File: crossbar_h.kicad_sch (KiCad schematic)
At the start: 64 parts, among them U100 AD5160, U101 AD5160, U102 AD5160, U103 AD5160, U104 AD5160, U105 AD5160, U106 AD5160, U107 AD5160, U108 AD5160, U109 AD5160, U110 AD5160, U111 AD5160, U112 AD5160, U113 AD5160, U114 AD5160, U115 AD5160, U116 AD5160, U117 AD5160, U118 AD5160, U119 AD5160, U120 AD5160, U121 AD5160, U122 AD5160, U123 AD5160, U124 AD5160, U125 AD5160, U126 AD5160, U127 AD5160, U128 AD5160, U129 AD5160, U130 AD5160, U131 AD5160

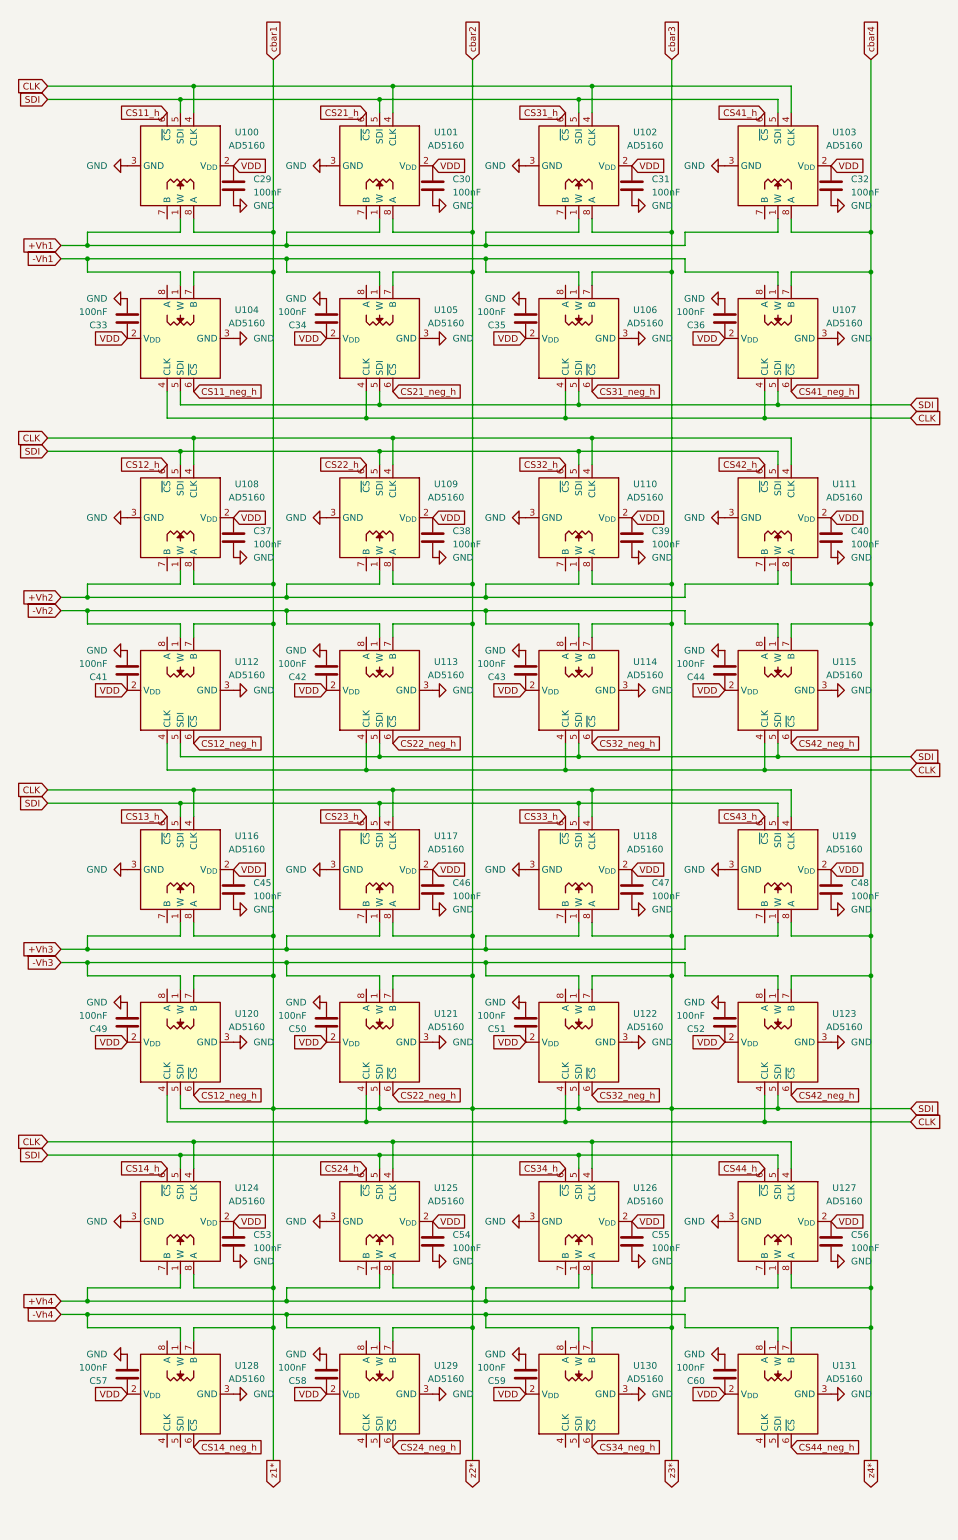
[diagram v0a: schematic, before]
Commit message: Updated: power
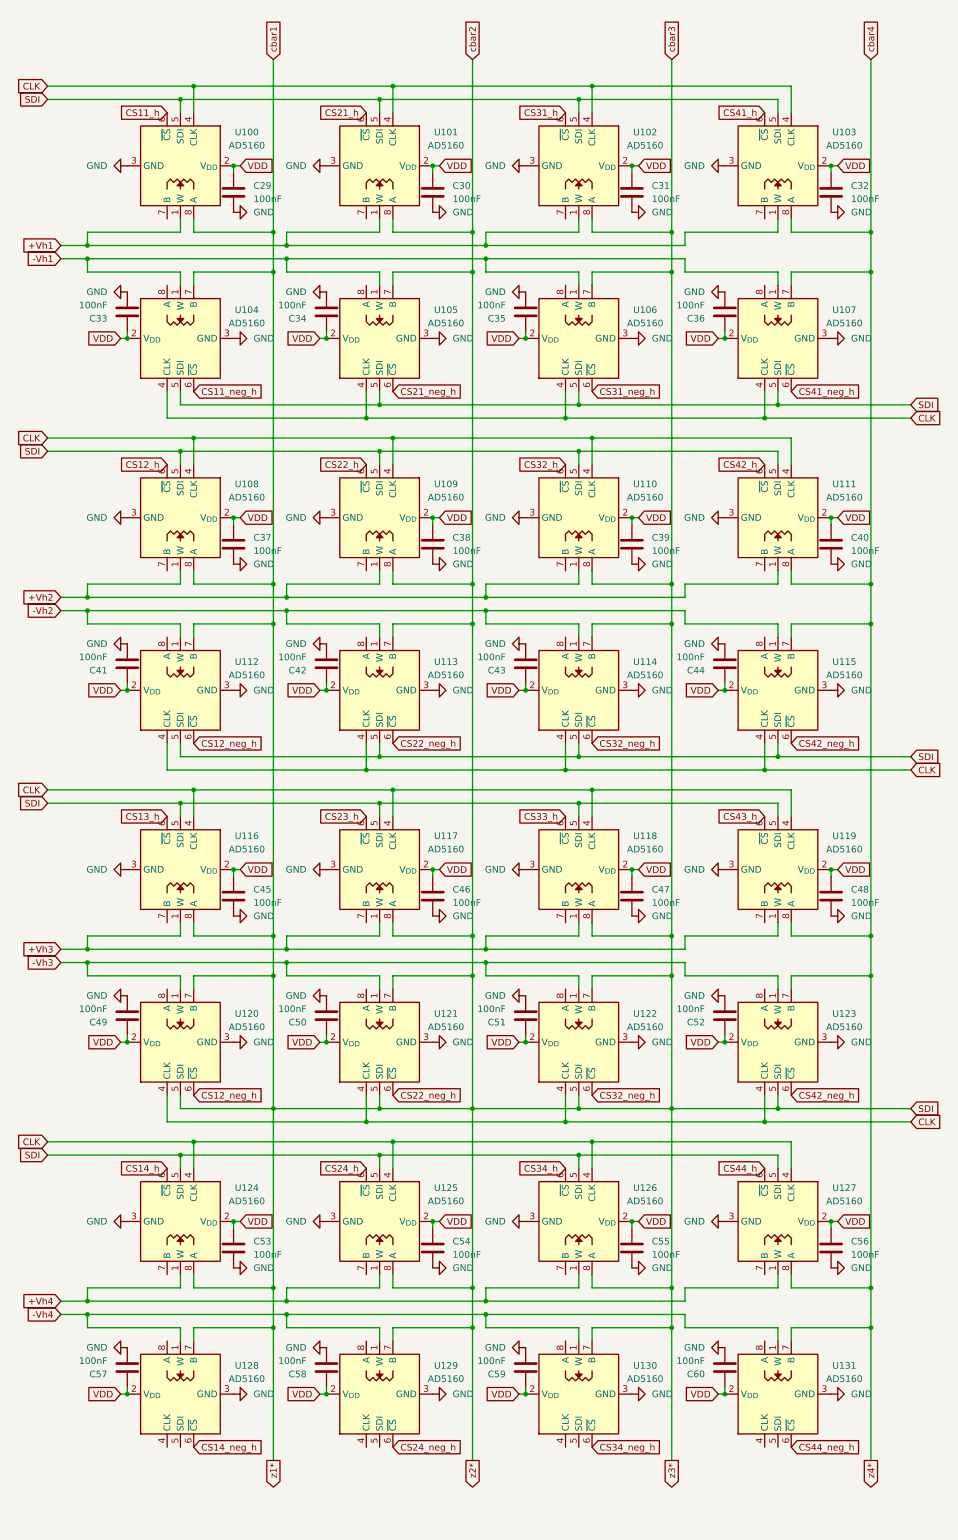
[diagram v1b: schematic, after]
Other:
- moved on the sheet: C29

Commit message: Updated: op amps
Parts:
- C29, C30, C31, C32, C33, C34, C35, C36, C37, C38, C39, C40, C41, C42, C43, C44, C45, C46, C47, C48, C49, C50, C51, C52, C53, C54, C55, C56, C57, C58, C59, C60: footprint (none) -> Capacitor_SMD:C_1206_3216Metric_Pad1.33x1.80mm_HandSolder
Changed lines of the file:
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@@
 			)
 		)
-		(property "Footprint" ""
+		(property "Footprint" "Capacitor_SMD:C_1206_3216Metric_Pad1.33x1.80mm_HandSolder"
 			(at 199.6948 240.03 0)
 			(effects
@@
 			)
 		)
-		(property "Footprint" ""
+		(property "Footprint" "Capacitor_SMD:C_1206_3216Metric_Pad1.33x1.80mm_HandSolder"
 			(at 221.9452 224.79 0)
 			(effects
@@
 			)
 		)
-		(property "Footprint" ""
+		(property "Footprint" "Capacitor_SMD:C_1206_3216Metric_Pad1.33x1.80mm_HandSolder"
 			(at 107.6452 90.17 0)
 			(effects
@@
 			)
 		)
-		(property "Footprint" ""
+		(property "Footprint" "Capacitor_SMD:C_1206_3216Metric_Pad1.33x1.80mm_HandSolder"
 			(at 199.6948 307.34 0)
 			(effects
@@
 			)
 		)
-		(property "Footprint" ""
+		(property "Footprint" "Capacitor_SMD:C_1206_3216Metric_Pad1.33x1.80mm_HandSolder"
 			(at 123.4948 240.03 0)
 			(effects
@@
 			)
 		)
-		(property "Footprint" ""
+		(property "Footprint" "Capacitor_SMD:C_1206_3216Metric_Pad1.33x1.80mm_HandSolder"
 			(at 199.6948 105.41 0)
 			(effects
@@
 			)
 		)
-		(property "Footprint" ""
+		(property "Footprint" "Capacitor_SMD:C_1206_3216Metric_Pad1.33x1.80mm_HandSolder"
 			(at 161.5948 307.34 0)
 			(effects
@@
 			)
 		)
-		(property "Footprint" ""
+		(property "Footprint" "Capacitor_SMD:C_1206_3216Metric_Pad1.33x1.80mm_HandSolder"
 			(at 85.3948 240.03 0)
 			(effects
@@
 			)
 		)
-		(property "Footprint" ""
+		(property "Footprint" "Capacitor_SMD:C_1206_3216Metric_Pad1.33x1.80mm_HandSolder"
 			(at 145.7452 292.1 0)
 			(effects
@@
 			)
 		)
-		(property "Footprint" ""
+		(property "Footprint" "Capacitor_SMD:C_1206_3216Metric_Pad1.33x1.80mm_HandSolder"
 			(at 145.7452 157.48 0)
 			(effects
@@
 			)
 		)
-		(property "Footprint" ""
+		(property "Footprint" "Capacitor_SMD:C_1206_3216Metric_Pad1.33x1.80mm_HandSolder"
 			(at 161.5948 172.72 0)
 			(effects
@@
 			)
 		)
-		(property "Footprint" ""
+		(property "Footprint" "Capacitor_SMD:C_1206_3216Metric_Pad1.33x1.80mm_HandSolder"
 			(at 183.8452 157.48 0)
 			(effects
@@
 			)
 		)
-		(property "Footprint" ""
+		(property "Footprint" "Capacitor_SMD:C_1206_3216Metric_Pad1.33x1.80mm_HandSolder"
 			(at 85.3948 307.34 0)
 			(effects
@@
 			)
 		)
-		(property "Footprint" ""
+		(property "Footprint" "Capacitor_SMD:C_1206_3216Metric_Pad1.33x1.80mm_HandSolder"
 			(at 107.6452 157.48 0)
 			(effects
@@
 			)
 		)
-		(property "Footprint" ""
+		(property "Footprint" "Capacitor_SMD:C_1206_3216Metric_Pad1.33x1.80mm_HandSolder"
 			(at 123.4948 172.72 0)
 			(effects
@@
 			)
 		)
-		(property "Footprint" ""
+		(property "Footprint" "Capacitor_SMD:C_1206_3216Metric_Pad1.33x1.80mm_HandSolder"
 			(at 199.6948 172.72 0)
 			(effects
@@
 			)
 		)
-		(property "Footprint" ""
+		(property "Footprint" "Capacitor_SMD:C_1206_3216Metric_Pad1.33x1.80mm_HandSolder"
 			(at 123.4948 105.41 0)
 			(effects
@@
 			)
 		)
-		(property "Footprint" ""
+		(property "Footprint" "Capacitor_SMD:C_1206_3216Metric_Pad1.33x1.80mm_HandSolder"
 			(at 145.7452 90.17 0)
 			(effects
@@
 			)
 		)
-		(property "Footprint" ""
+		(property "Footprint" "Capacitor_SMD:C_1206_3216Metric_Pad1.33x1.80mm_HandSolder"
 			(at 183.8452 224.79 0)
 			(effects
@@
 			)
 		)
-		(property "Footprint" ""
+		(property "Footprint" "Capacitor_SMD:C_1206_3216Metric_Pad1.33x1.80mm_HandSolder"
 			(at 183.8452 292.1 0)
 			(effects
@@
 			)
 		)
-		(property "Footprint" ""
+		(property "Footprint" "Capacitor_SMD:C_1206_3216Metric_Pad1.33x1.80mm_HandSolder"
 			(at 145.7452 224.79 0)
 			(effects
@@
 			)
 		)
-		(property "Footprint" ""
+		(property "Footprint" "Capacitor_SMD:C_1206_3216Metric_Pad1.33x1.80mm_HandSolder"
 			(at 107.6452 224.79 0)
 			(effects
@@
 			)
 		)
-		(property "Footprint" ""
+		(property "Footprint" "Capacitor_SMD:C_1206_3216Metric_Pad1.33x1.80mm_HandSolder"
 			(at 183.8452 90.17 0)
 			(effects
@@
 			)
 		)
-		(property "Footprint" ""
+		(property "Footprint" "Capacitor_SMD:C_1206_3216Metric_Pad1.33x1.80mm_HandSolder"
 			(at 161.5948 240.03 0)
 			(effects
@@
 			)
 		)
-		(property "Footprint" ""
+		(property "Footprint" "Capacitor_SMD:C_1206_3216Metric_Pad1.33x1.80mm_HandSolder"
 			(at 221.9452 292.1 0)
 			(effects
@@
 			)
 		)
-		(property "Footprint" ""
+		(property "Footprint" "Capacitor_SMD:C_1206_3216Metric_Pad1.33x1.80mm_HandSolder"
 			(at 221.9452 157.48 0)
 			(effects
@@
 			)
 		)
-		(property "Footprint" ""
+		(property "Footprint" "Capacitor_SMD:C_1206_3216Metric_Pad1.33x1.80mm_HandSolder"
 			(at 221.9452 90.17 0)
 			(effects
@@
 			)
 		)
-		(property "Footprint" ""
+		(property "Footprint" "Capacitor_SMD:C_1206_3216Metric_Pad1.33x1.80mm_HandSolder"
 			(at 107.6452 292.1 0)
 			(effects
@@
 			)
 		)
-		(property "Footprint" ""
+		(property "Footprint" "Capacitor_SMD:C_1206_3216Metric_Pad1.33x1.80mm_HandSolder"
 			(at 85.3948 105.41 0)
 			(effects
@@
 			)
 		)
-		(property "Footprint" ""
+		(property "Footprint" "Capacitor_SMD:C_1206_3216Metric_Pad1.33x1.80mm_HandSolder"
 			(at 161.5948 105.41 0)
 			(effects
@@
 			)
 		)
-		(property "Footprint" ""
+		(property "Footprint" "Capacitor_SMD:C_1206_3216Metric_Pad1.33x1.80mm_HandSolder"
 			(at 123.4948 307.34 0)
 			(effects
@@
 			)
 		)
-		(property "Footprint" ""
+		(property "Footprint" "Capacitor_SMD:C_1206_3216Metric_Pad1.33x1.80mm_HandSolder"
 			(at 85.3948 172.72 0)
 			(effects

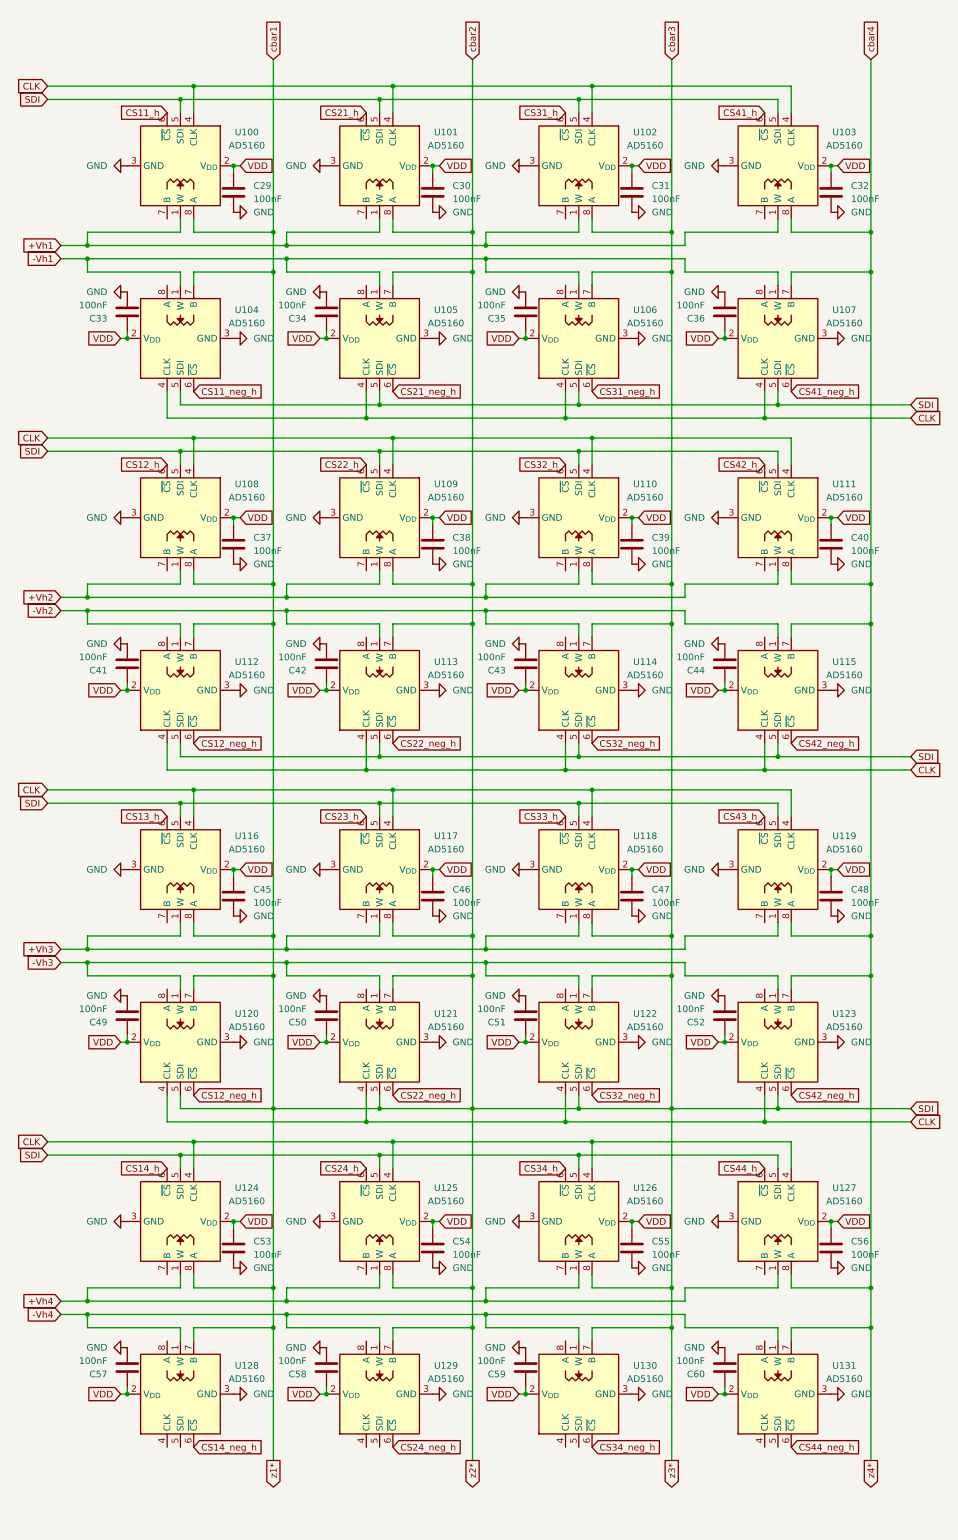
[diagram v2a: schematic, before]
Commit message: Updated: pots
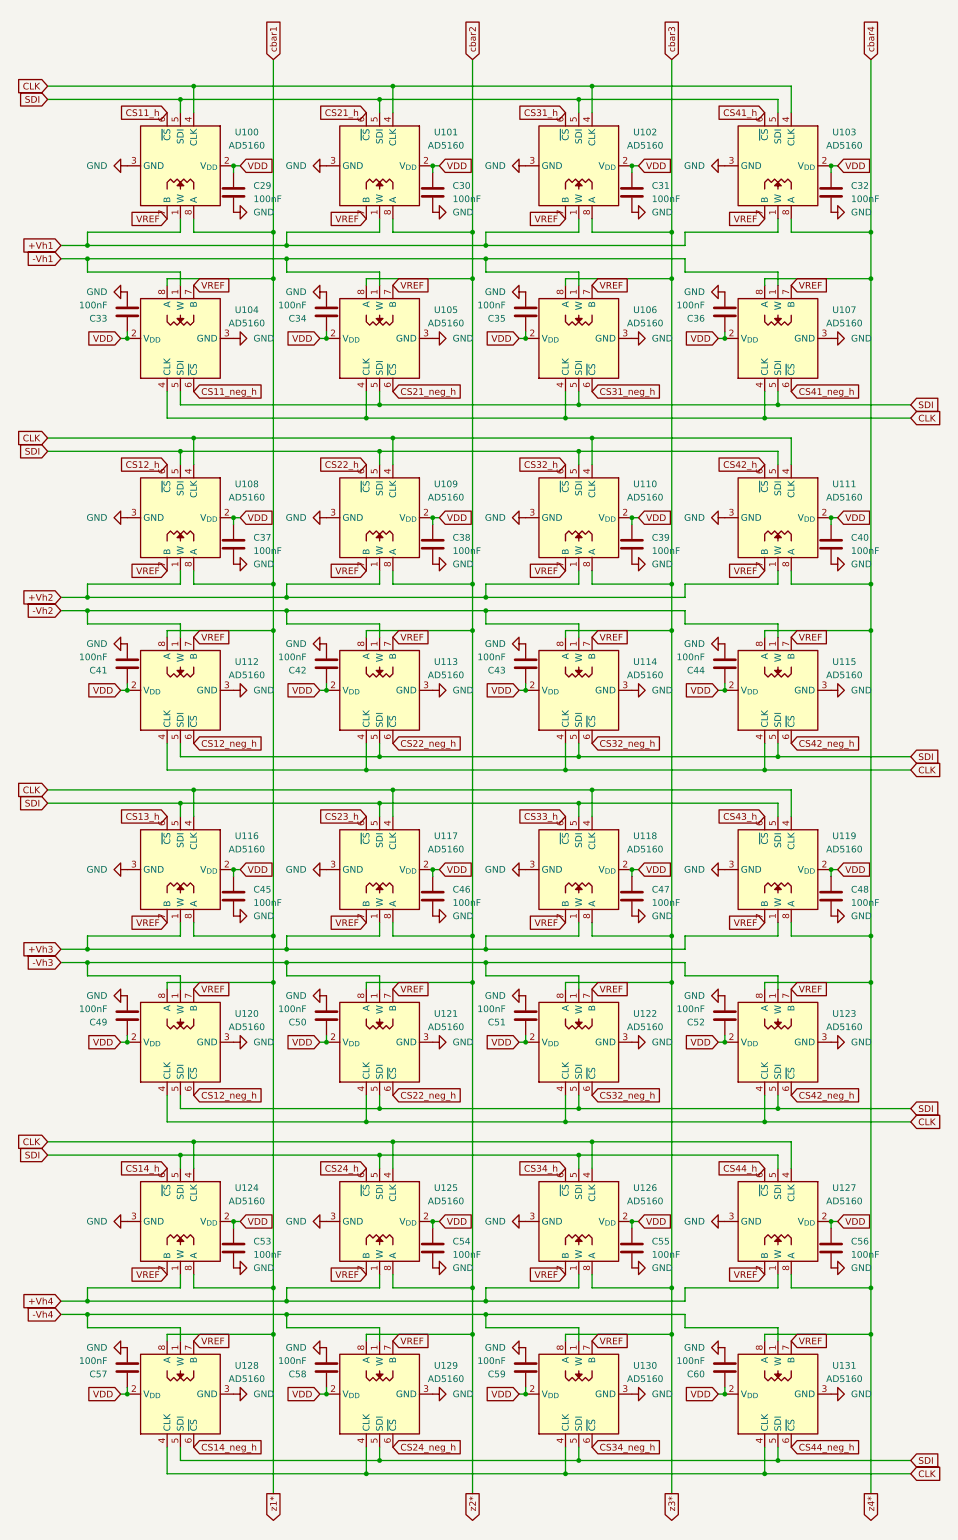
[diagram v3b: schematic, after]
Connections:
- net CLK: now also U128.4 (CLK), U129.4 (CLK), U130.4 (CLK), U131.4 (CLK)
- net SDI: now also U128.5 (SDI), U129.5 (SDI), U130.5 (SDI), U131.5 (SDI); no longer U100.8 (A), U101.8 (A), U102.8 (A), U104.7 (B), U105.7 (B), U106.7 (B), U108.8 (A), U109.8 (A), U110.8 (A), U112.7 (B), U113.7 (B), U114.7 (B), U116.8 (A), U117.8 (A), U118.8 (A), U120.7 (B), U121.7 (B), U122.7 (B), U124.8 (A), U125.8 (A), U126.8 (A), U128.7 (B), U129.7 (B), U130.7 (B)
- net cbar4: now also U107.8 (A), U115.8 (A), U123.8 (A), U131.8 (A); no longer U107.7 (B), U115.7 (B), U123.7 (B), U131.7 (B)
- net VREF: now reaches U126.7 (B)
- net VREF: now also U100.7 (B), U101.7 (B), U102.7 (B), U103.7 (B), U104.7 (B), U105.7 (B), U106.7 (B), U107.7 (B), U108.7 (B), U109.7 (B), U110.7 (B), U111.7 (B), U112.7 (B), U113.7 (B), U114.7 (B), U115.7 (B), U116.7 (B), U117.7 (B), U118.7 (B), U119.7 (B), U120.7 (B), U121.7 (B), U122.7 (B), U123.7 (B), U124.7 (B), U125.7 (B), U127.7 (B), U128.7 (B), U129.7 (B), U130.7 (B), U131.7 (B)
- net cbar1: now reaches U128.8 (A)
- net cbar1: now also U100.8 (A), U104.8 (A), U108.8 (A), U112.8 (A), U116.8 (A), U120.8 (A), U124.8 (A)
- net cbar3: now reaches U114.8 (A)
- net cbar3: now also U102.8 (A), U106.8 (A), U110.8 (A), U118.8 (A), U122.8 (A), U126.8 (A), U130.8 (A)
- net cbar2: now reaches U121.8 (A)
- net cbar2: now also U101.8 (A), U105.8 (A), U109.8 (A), U113.8 (A), U117.8 (A), U125.8 (A), U129.8 (A)
